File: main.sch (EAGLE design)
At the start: 39 parts, among them IC1 ATTINY13A-SSH, IC2 TP4056-42-ESOP8, IC3 LM27313XMFX_NOPB, IC4 TPL5110DDCT, T1A 2N4401, T1B NPN, X1 MINI-USB-UX60A-MB-5ST, X2 332-02

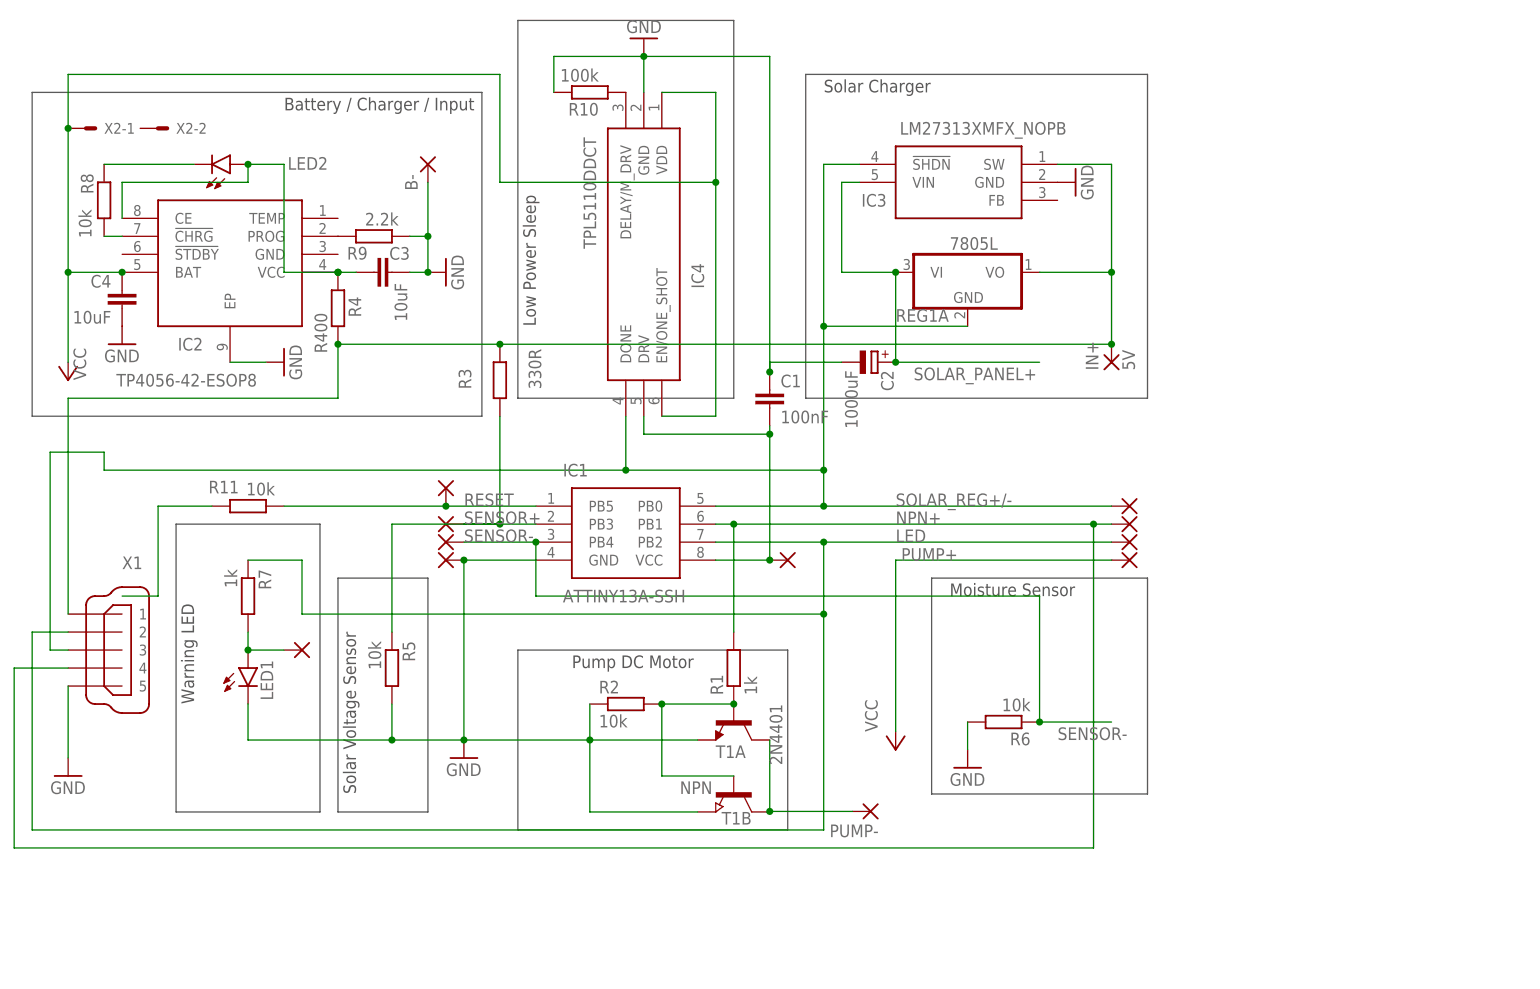
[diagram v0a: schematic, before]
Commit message: rev 0.8 (usbtiny built-in)
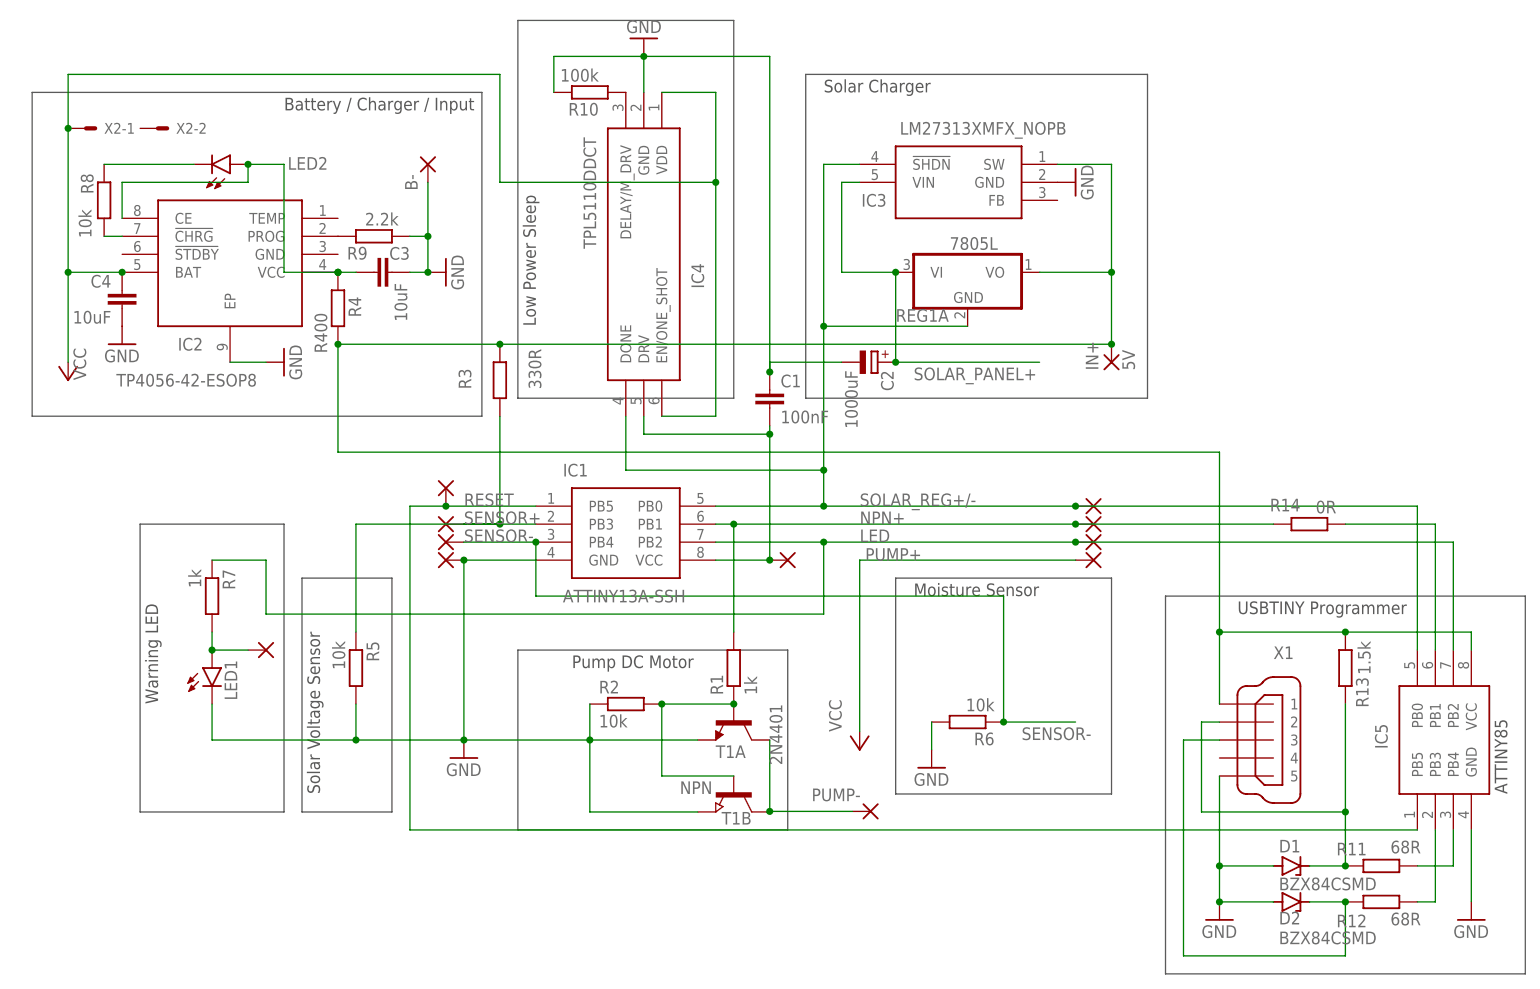
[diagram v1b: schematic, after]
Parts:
- added D1, D2: BZX84CSMD, diode:BZX84CSMD
- added IC5: ATTINY13A-SSH, STM32F103RBT6:ATTINY13A-SSH
- added R12: 68R, resistor:R-EU_R0603
- added R13: 1.5k, resistor:R-EU_R0603
- added R14: 0R, resistor:R-EU_R0402
- C4: device rcl:C-EUC3216 -> rcl:C-EUC1206
- R11: value 10k -> 68R
- R7: device resistor:R-EU_M0805 -> resistor:R-EU_R0603
- R9: device rcl:R-EU_R0805 -> rcl:R-EU_R0603
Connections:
- new net N$10: IC5.PB4, R11.2
- new net N$13: D1.C, R11.1, R13.2, X1.2
- new net N$14: D2.C, R12.1, X1.3
- new net N$15: IC5.PB1, R14.1
- net GND: now also D1.A, D2.A, IC5.GND
- net LED: now also IC5.PB2; no longer X1.2
- net N$12: now also IC5.PB3, R12.2; no longer R11.2
- net N$5: now also IC5.VCC, R13.1
- net NPN+: now also R14.2; no longer X1.4
- net RESET: now also IC5.PB5; no longer R11.1
- net SOLAR_REG+/-: now also IC5.PB0; no longer X1.3
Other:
- note added: "ATTINY85"
- note added: "USBTINY Programmer"
- moved on the sheet: LED1, PUMP+, R11, R5, R6, R7, X1
